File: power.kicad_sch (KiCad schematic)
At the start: 25 parts, among them J1 Conn_01x06_Pin, U13 LP5907MFX-3.0, U15 LP5907MFX-3.0, U3 LM66100DCK, U5 TPS22918TDBVRQ1, U6 LP5907MFX-3.0

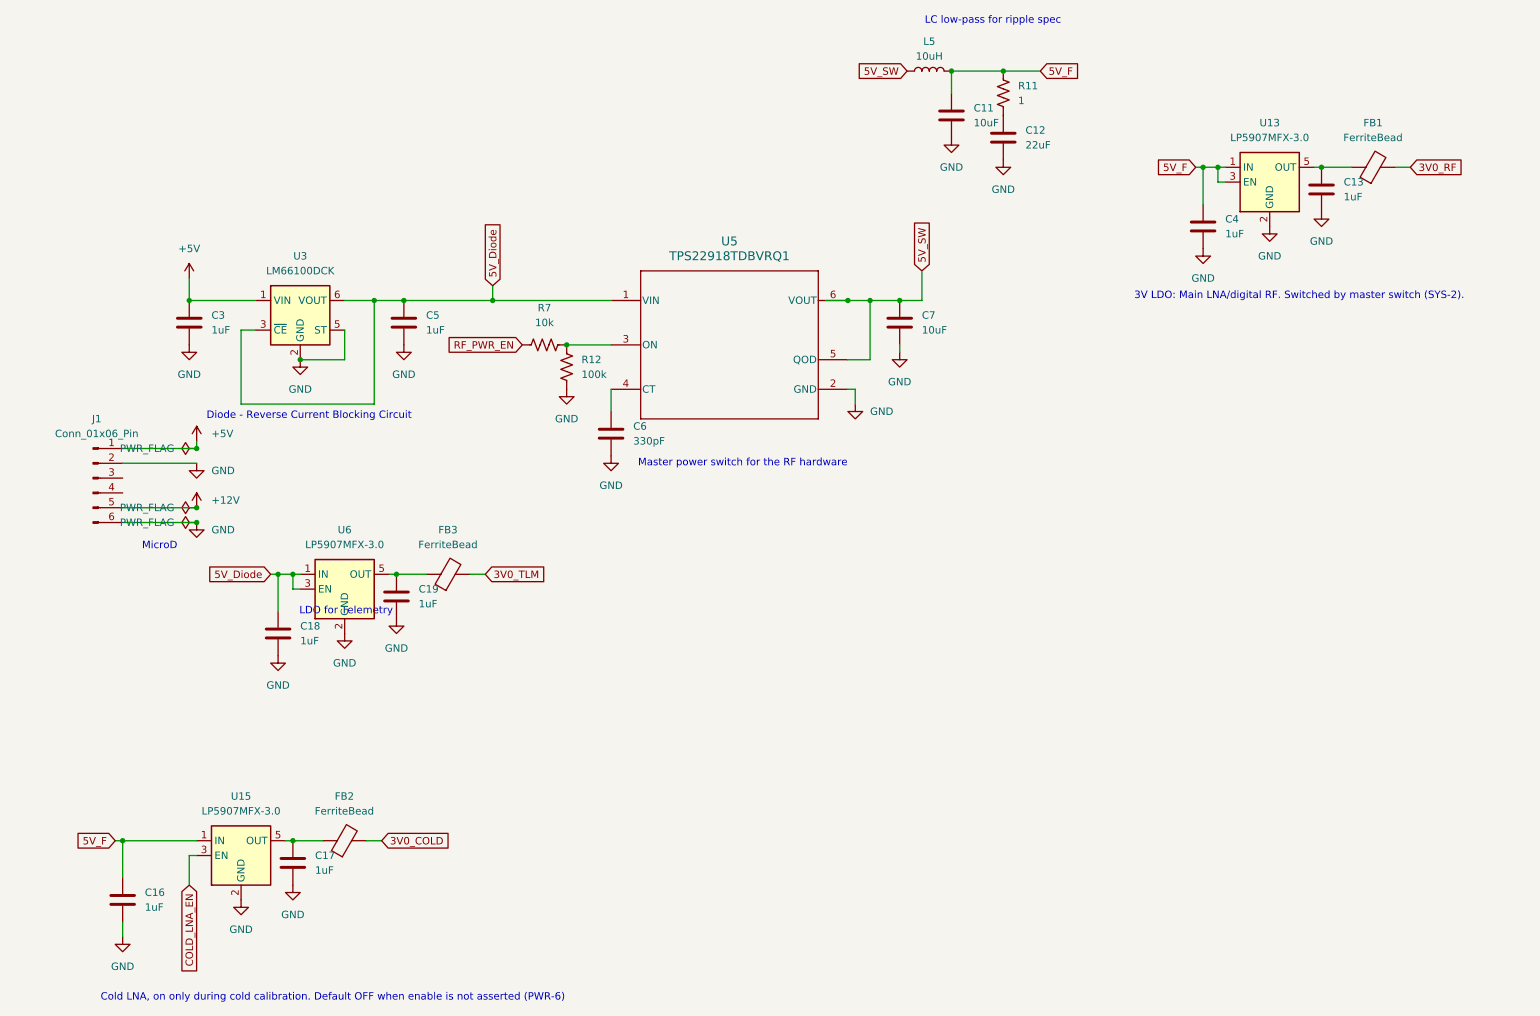
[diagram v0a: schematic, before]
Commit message: 12V_F
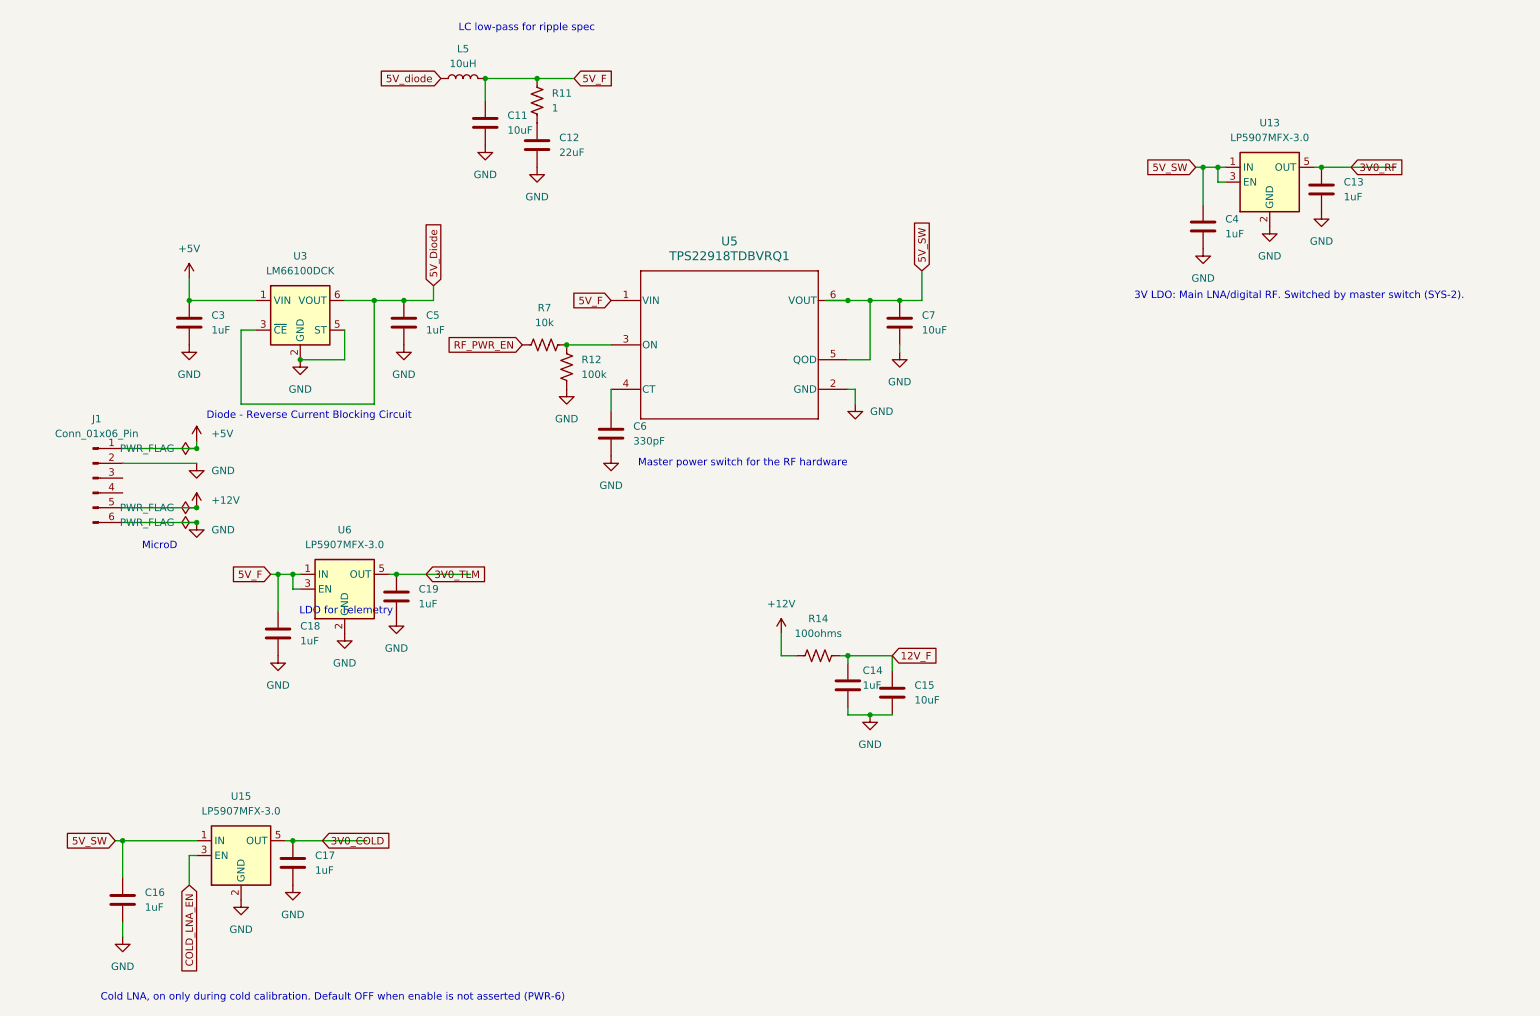
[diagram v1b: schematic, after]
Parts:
- removed FB1, FB2, FB3: FerriteBead, symbol Device:FerriteBead
- added C14: 1uF, symbol Device:C
- added C15: 10uF, symbol Device:C
- added R14: 100ohms, symbol Device:R_US
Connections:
- net +12V: now also R14.1
- net 3V0_COLD: now also C17.1, U15.5 (OUT)
- net 3V0_RF: now also C13.1, U13.5 (OUT)
- net 3V0_TLM: now also C19.1, U6.5 (OUT)
- net 5V_Diode: no longer C18.1, U5.1 (VIN), U6.1 (IN), U6.3 (EN)
- net 5V_F: now also C18.1, U5.1 (VIN), U6.1 (IN), U6.3 (EN); no longer C16.1, C4.1, U13.1 (IN), U13.3 (EN), U15.1 (IN)
- net 5V_SW: now also C16.1, C4.1, U13.1 (IN), U13.3 (EN), U15.1 (IN); no longer L5.1
- net GND: now also C14.2, C15.2
- new net 12V_F: C14.1, C15.1, R14.2
- new net 5V_diode: L5.1
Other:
- moved on the sheet: C11, C12, L5, R11
